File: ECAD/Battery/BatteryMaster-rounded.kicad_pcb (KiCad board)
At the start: 2 copper layers, 90.2 x 95.9 mm, 149 parts, among them J1 SWD/DEBUG, Q1 DMP3015LSSQ, Q10 DMP3015LSSQ, Q11 DMP3015LSSQ, Q12 DMP3015LSSQ, Q13 Si4186DY, Q14 DMP3015LSSQ, Q15 Si4186DY, Q16 2N7002, Q17 Si2371EDS-T1-BE3, Q18 DMG6968U-7, Q19 2N7002, Q2 Si4186DY, Q20 Si2371EDS-T1-BE3, Q21 DMG6968U-7, Q22 2N7002, Q23 Si2371EDS-T1-BE3, Q24 DMG6968U-7, Q25 2N7002, Q26 Si2371EDS-T1-BE3, Q27 DMG6968U-7, Q3 2N7002, Q4 DMP3015LSSQ, Q5 DMP3015LSSQ, Q6 2N7002, Q7 DMP3015LSSQ, Q8 DMP3015LSSQ, Q9 Si4186DY, SW1 INHIBIT, SW2 INHIBIT, SW3 INHIBIT, SW4 INHIBIT, SW5 INHIBIT, U1 LM1117-3.3, U10 BQ29209, U2 LTC4359-MS8, U3 INA181A2, U4 MAX6035xxUR30, U5 LM358, U6 TLV9361IDBVR, U7 MAX6369, U8 LTC4365TS8-1, U9 STM32F103C8Tx, Y1 8MHz

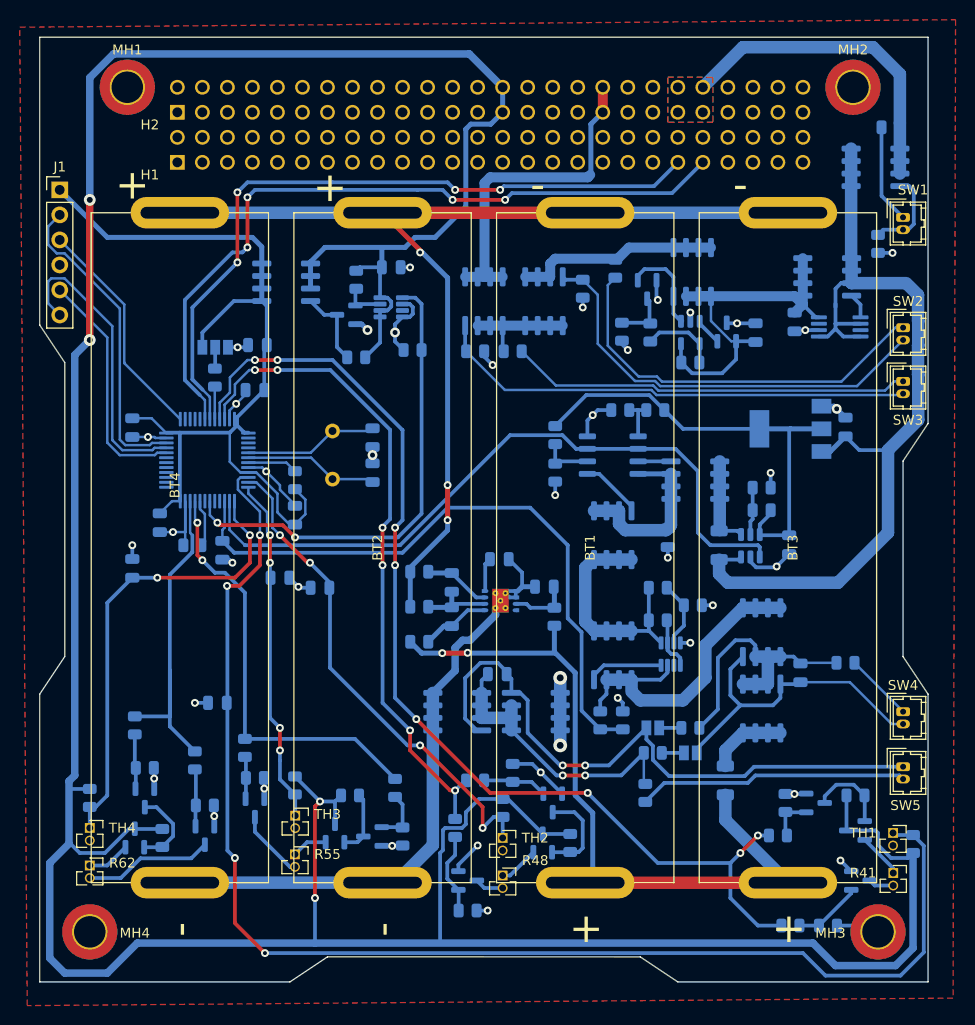
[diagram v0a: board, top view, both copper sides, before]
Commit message: finish battery
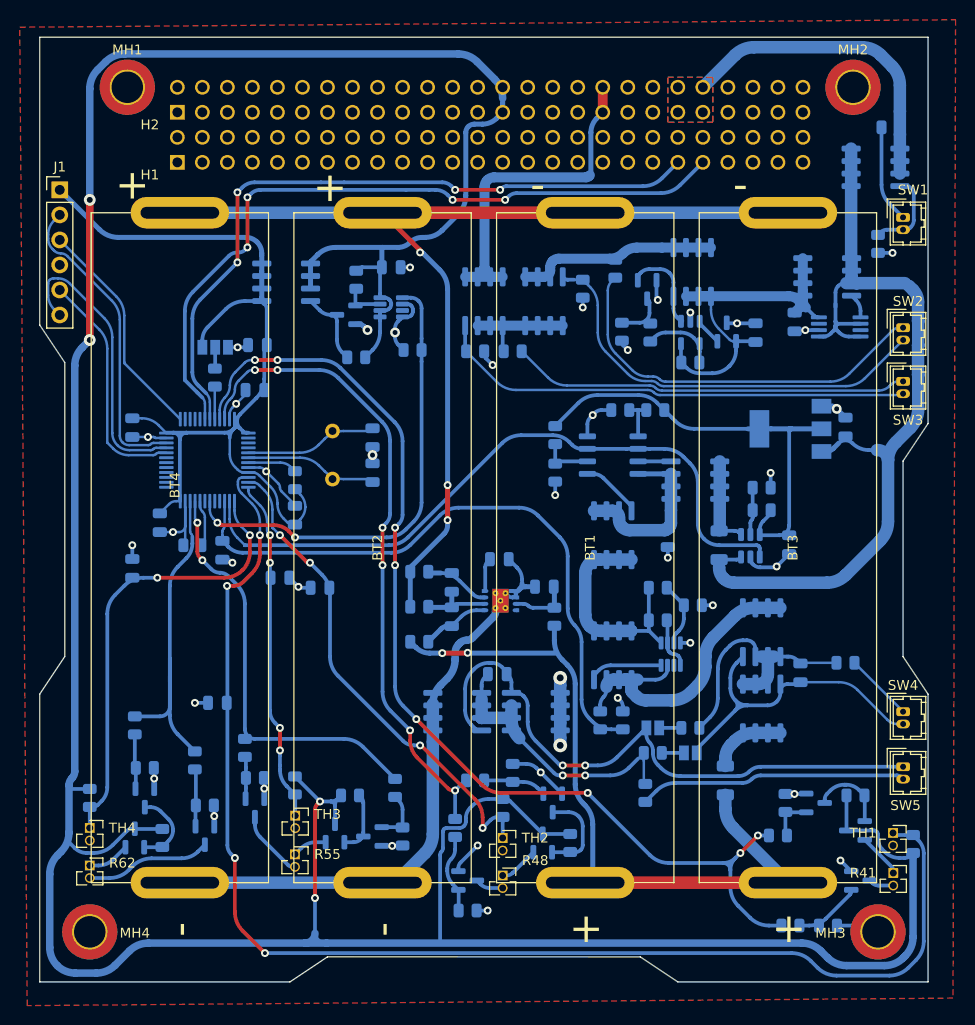
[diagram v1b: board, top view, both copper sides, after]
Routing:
- net Net-(C1-Pad1): track 91.4 -> 94.3 mm
- net VDD: track 92.2 -> 94.9 mm
- net GND: track 112.2 -> 109.7 mm
- net Net-(C15-Pad1): track 64.1 -> 61.9 mm
- net PCM_IN: track 33.8 -> 35.5 mm
- net +3V3: track 364.5 -> 363.2 mm
- net /TBAT1: track 137.1 -> 135.8 mm
- net Net-(C12-Pad1): track 27.7 -> 26.4 mm
- net Net-(C15-Pad2): track 29.8 -> 28.5 mm
- net /TELEM_VBAT: track 65.5 -> 64.3 mm
- net Net-(BT1-Pad2): track 106.1 -> 105.0 mm
- net /TELEM_IBAT: track 72.9 -> 71.8 mm
- net /TBAT2: track 51.0 -> 50.1 mm
- net /H3CTRL: track 43.7 -> 42.8 mm
- net /TBAT4: track 47.0 -> 46.1 mm
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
